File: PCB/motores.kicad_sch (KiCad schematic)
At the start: 30 parts, among them IC2 IR2175STRPBF, J10 Conn_01x03, J11 Conn_01x03, J12 motor_dc, J9 motor_lineal, K1 G6E, K2 G6E, K3 G6E, K4 G6E, Q1 AO3401A, Q2 AO3401A, Q3 AO3401A, Q4 AO3401A

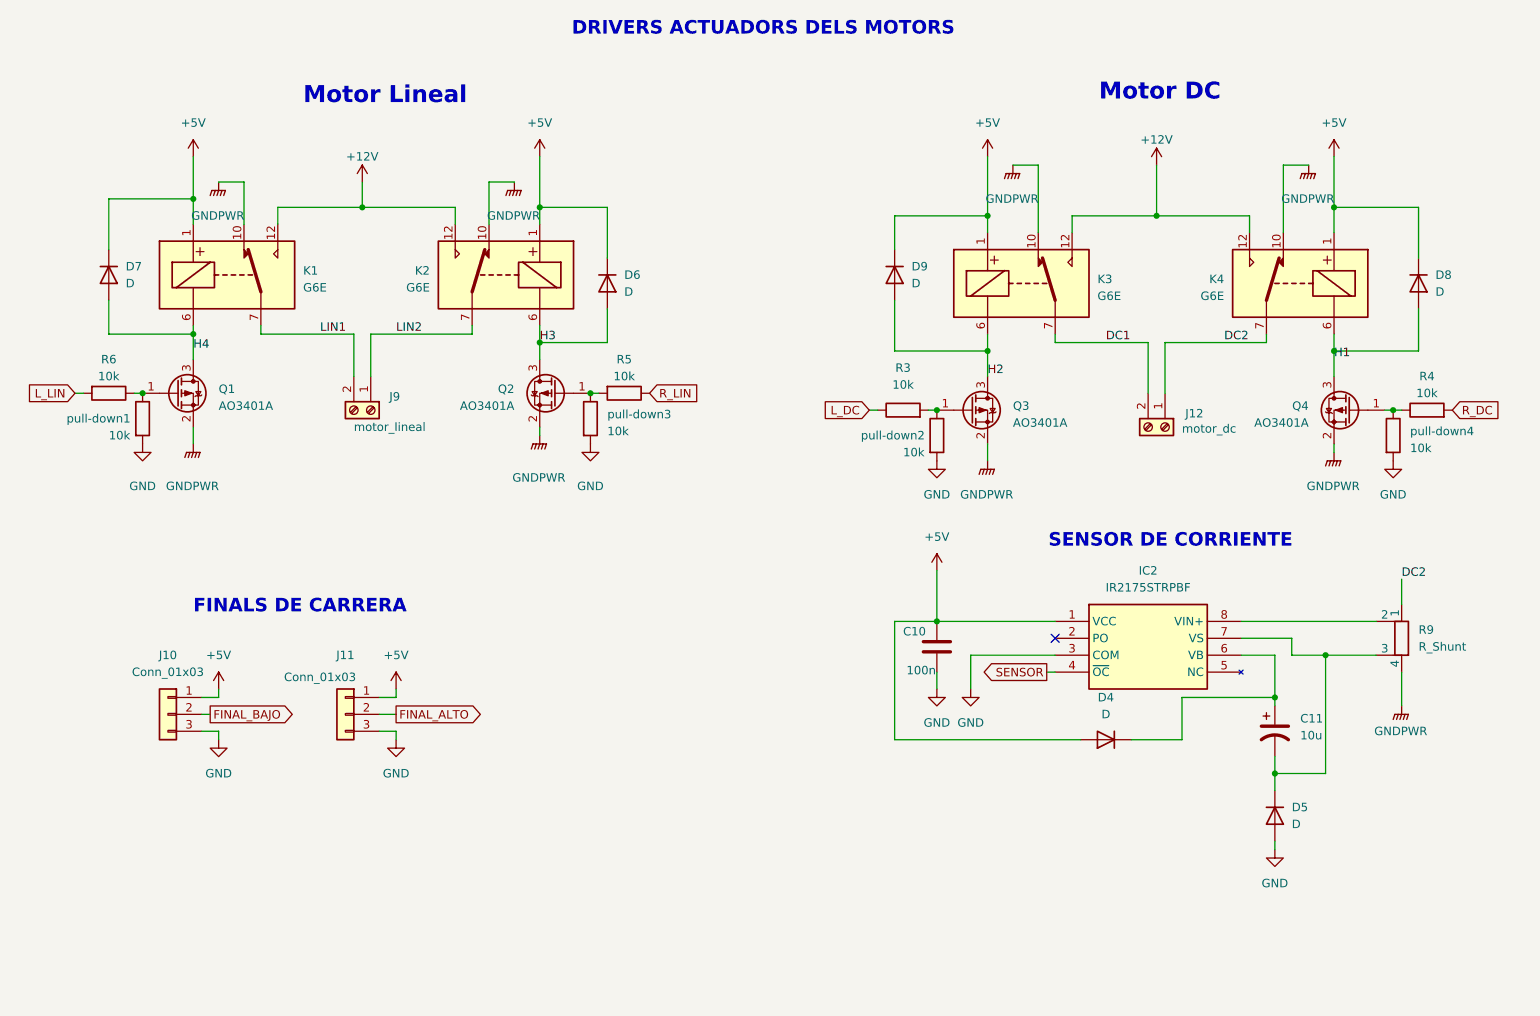
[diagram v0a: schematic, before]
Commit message: esquemático  v2
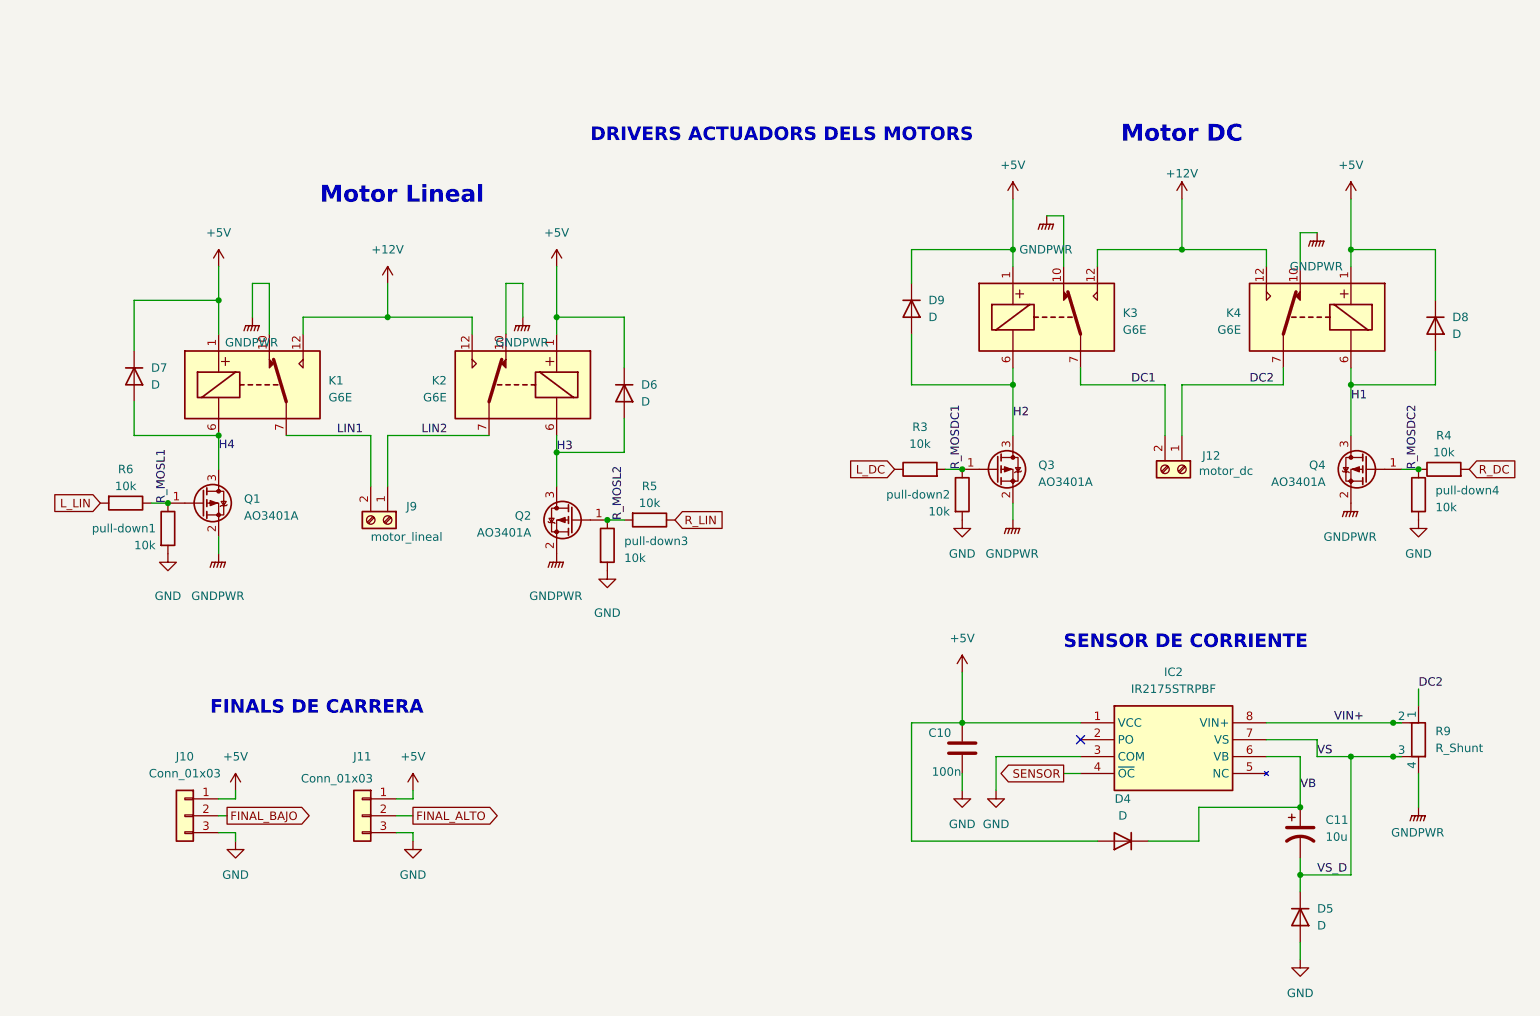
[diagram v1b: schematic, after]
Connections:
- net R_MOSDC2: now reaches Q4.1 (G), R4.1, pull-down4.1
- net R_MOSL1: now reaches Q1.1 (G), R6.1, pull-down1.1
- net VS: now reaches C11.2, D5.1 (K), IC2.7 (VS), R9.3
- net R_MOSL2: now reaches Q2.1 (G), R5.2, pull-down3.1
- net R_MOSDC1: now reaches Q3.1 (G), R3.2, pull-down2.1
- net VIN+: now reaches IC2.8 (VIN+), R9.2
- net VB: now reaches C11.1, D4.1 (K), IC2.6 (VB)
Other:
- moved on the sheet: C10, C11, D4, D5, D6, D7, D8, D9, IC2, J10, J11, J12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
